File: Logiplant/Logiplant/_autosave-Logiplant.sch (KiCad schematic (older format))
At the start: 18 parts, among them J4 POWER, J6 Conn_RELE, J7 Conn_IMPRESOR, U2 ESP32-DEVKITC-32D

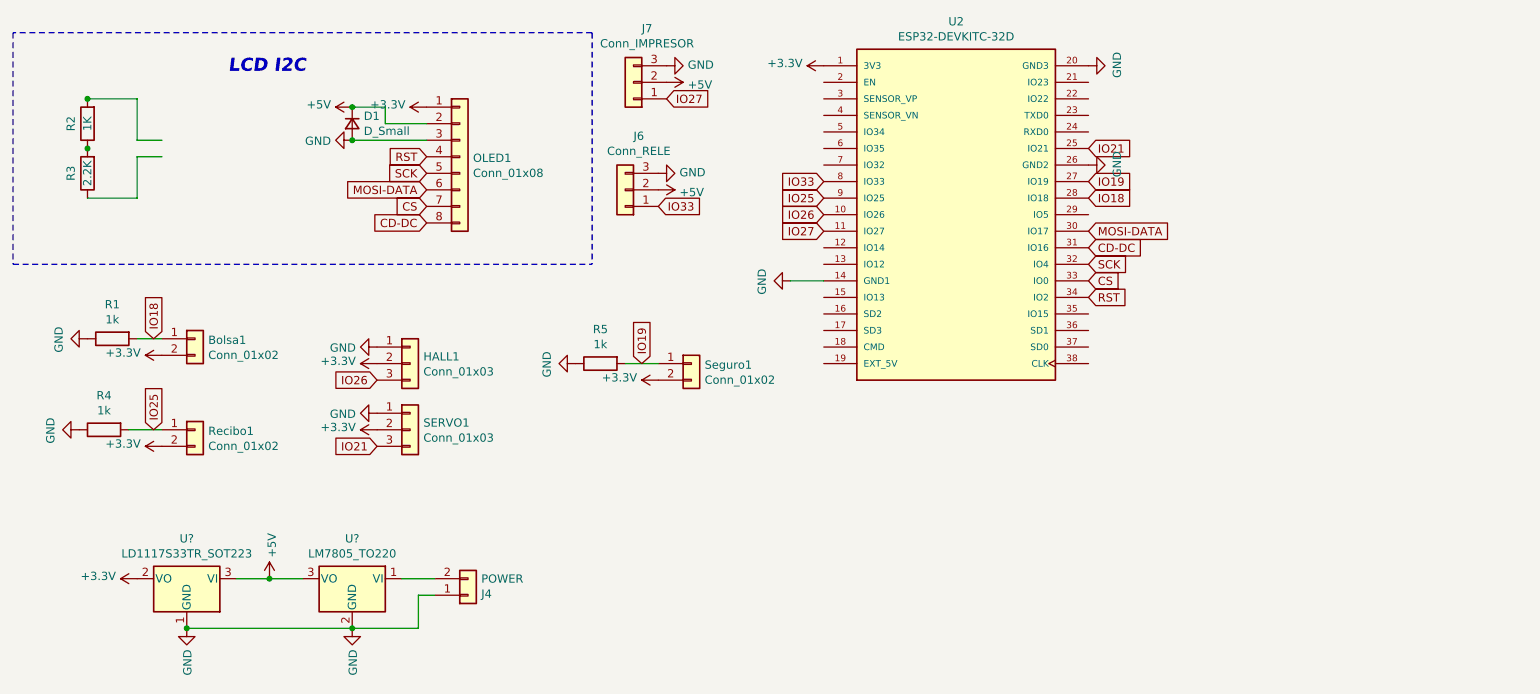
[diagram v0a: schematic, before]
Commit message: Nueva regulación
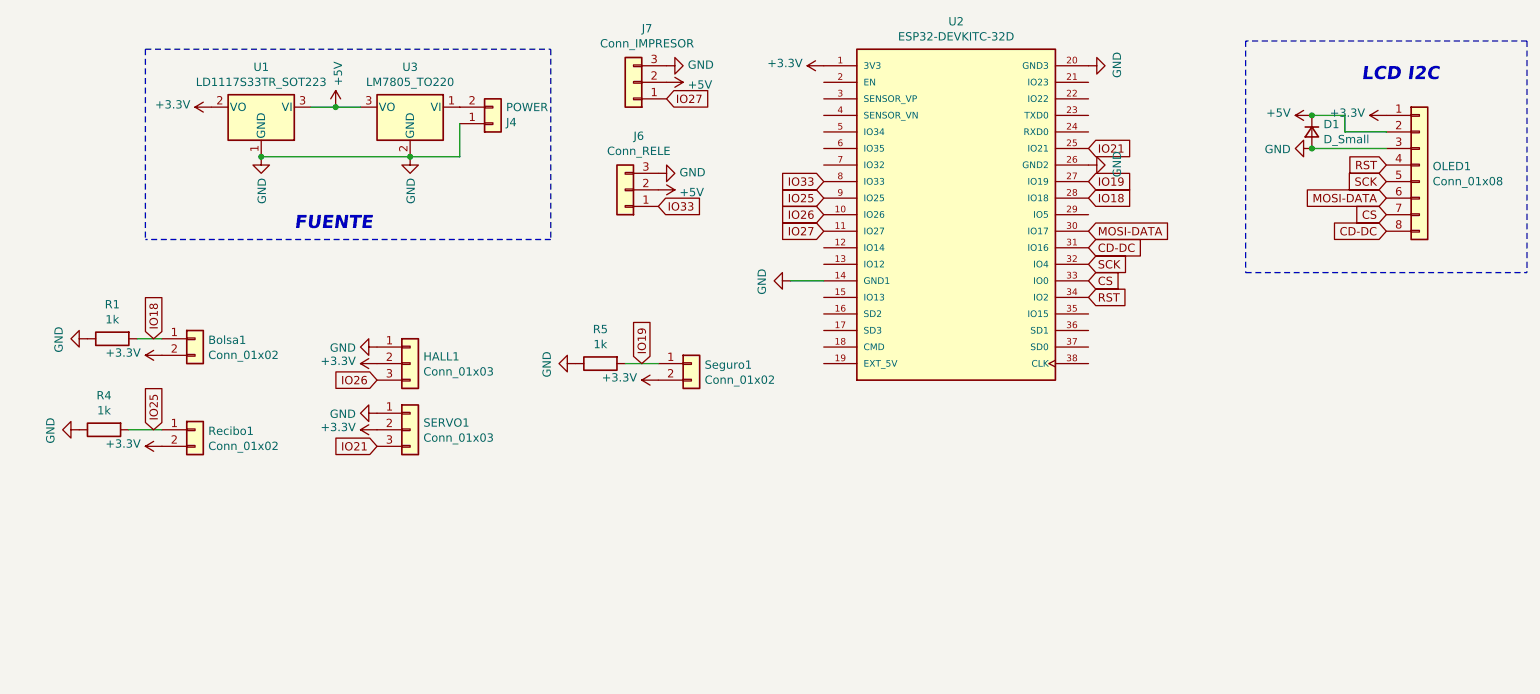
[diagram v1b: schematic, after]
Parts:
- removed R2: 1K, Resistor_THT:R_Axial_DIN0207_L6.3mm_D2.5mm_P5.08mm_Vertical, symbol Device:R
- removed R3: 2.2K, Resistor_THT:R_Axial_DIN0207_L6.3mm_D2.5mm_P5.08mm_Vertical, symbol Device:R
- U1: renamed from U?; footprint Package_TO_SOT_SMD:SOT-223-3_TabPin2 -> Package_TO_SOT_THT:TO-220-3_Vertical
- gave numbers to parts that had none: 1
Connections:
- wire segments 21 -> 13
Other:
- note added: "FUENTE"
- moved on the sheet: D1, J4, OLED1, U1, U3
